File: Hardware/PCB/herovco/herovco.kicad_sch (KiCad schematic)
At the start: 19 parts, among them J1 Conn_01x09, J10 Conn_01x09, J11 Conn_01x06, J12 Conn_01x03, J13 Conn_01x03, J14 3_pin_Molex_connector, J15 Wire pads, J16 Conn_01x01, J17 Conn_01x01, J18 Conn_01x01, J19 Conn_02x04_Odd_Even, J2 Conn_01x06, J3 Conn_01x03, J4 Conn_01x03, J5 3_pin_Molex_header, J6 Wire pads, J7 Conn_01x01, J8 Conn_01x01, J9 Conn_01x01

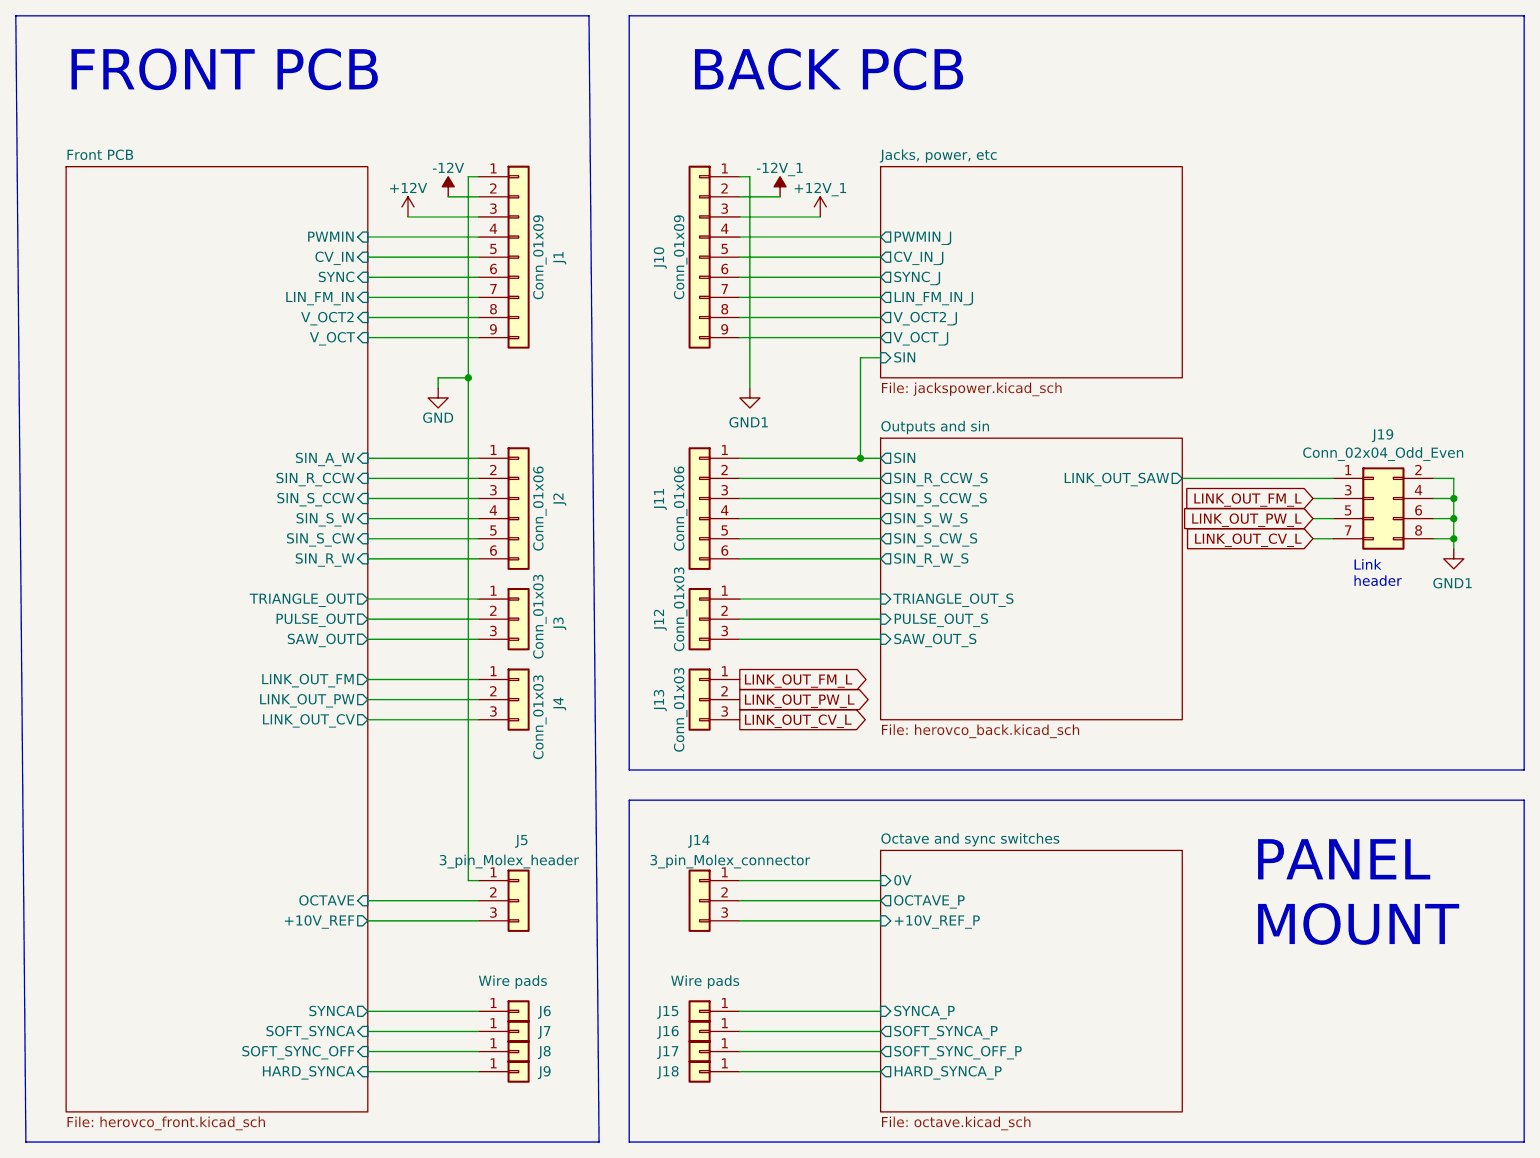
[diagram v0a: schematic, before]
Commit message: Sine trimmers to back board, misc accumulated tweaks
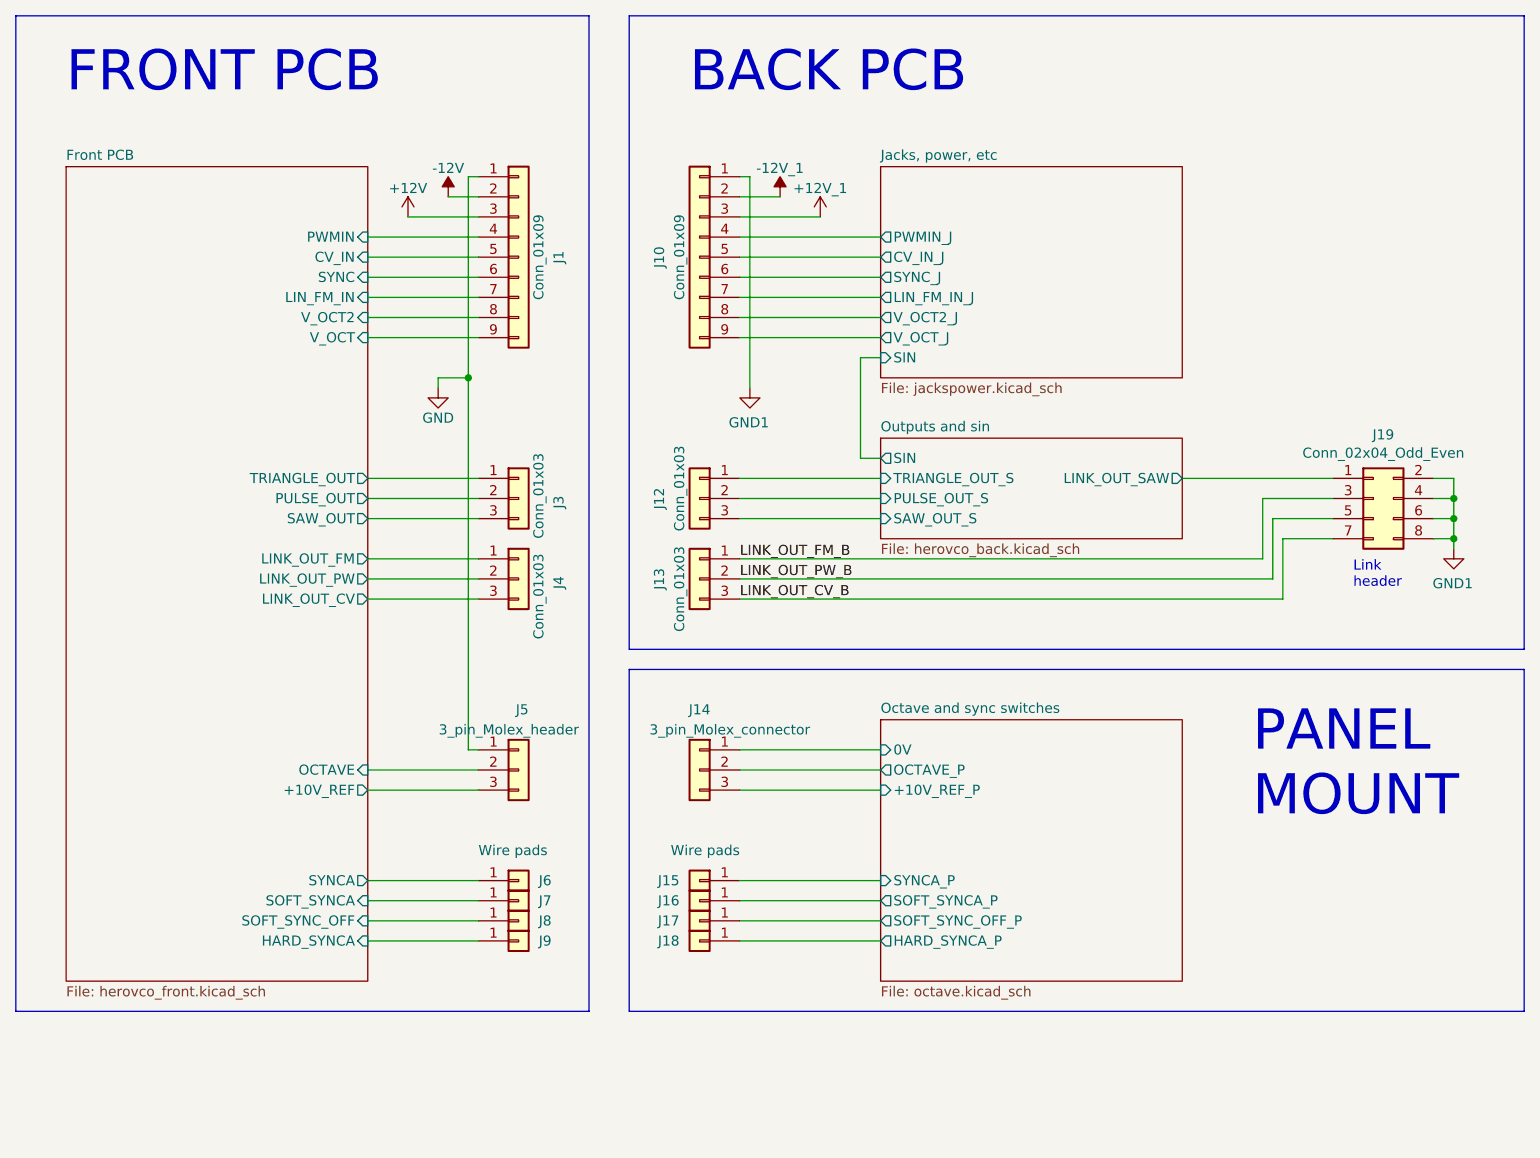
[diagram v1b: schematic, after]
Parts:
- removed J11: Conn_01x06, Connector_PinSocket_2.54mm:PinSocket_1x06_P2.54mm_Vertical, symbol Connector_Generic:Conn_01x06
- removed J2: Conn_01x06, Connector_PinHeader_2.54mm:PinHeader_1x06_P2.54mm_Vertical, symbol Connector_Generic:Conn_01x06
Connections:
- net LINK_OUT_CV_L renamed LINK_OUT_CV_B
- net LINK_OUT_FM_L renamed LINK_OUT_FM_B
- net LINK_OUT_PW_L renamed LINK_OUT_PW_B
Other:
- sheet Front PCB ports: added none; removed SIN_A_W, SIN_R_CCW, SIN_R_W, SIN_S_CCW, SIN_S_CW, SIN_S_W
- sheet Outputs and sin ports: added none; removed SIN_R_CCW_S, SIN_R_W_S, SIN_S_CCW_S, SIN_S_CW_S, SIN_S_W_S
- moved on the sheet: J12, J13, J14, J15, J16, J17, J18, J3, J4, J5, J6, J7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
